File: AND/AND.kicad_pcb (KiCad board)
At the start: 2 copper layers, 33.7 x 17.8 mm, 9 parts, among them J1 Conn_01x01, J2 Conn_01x01, J3 Conn_01x01, J4 Conn_01x01, J5 Conn_01x02

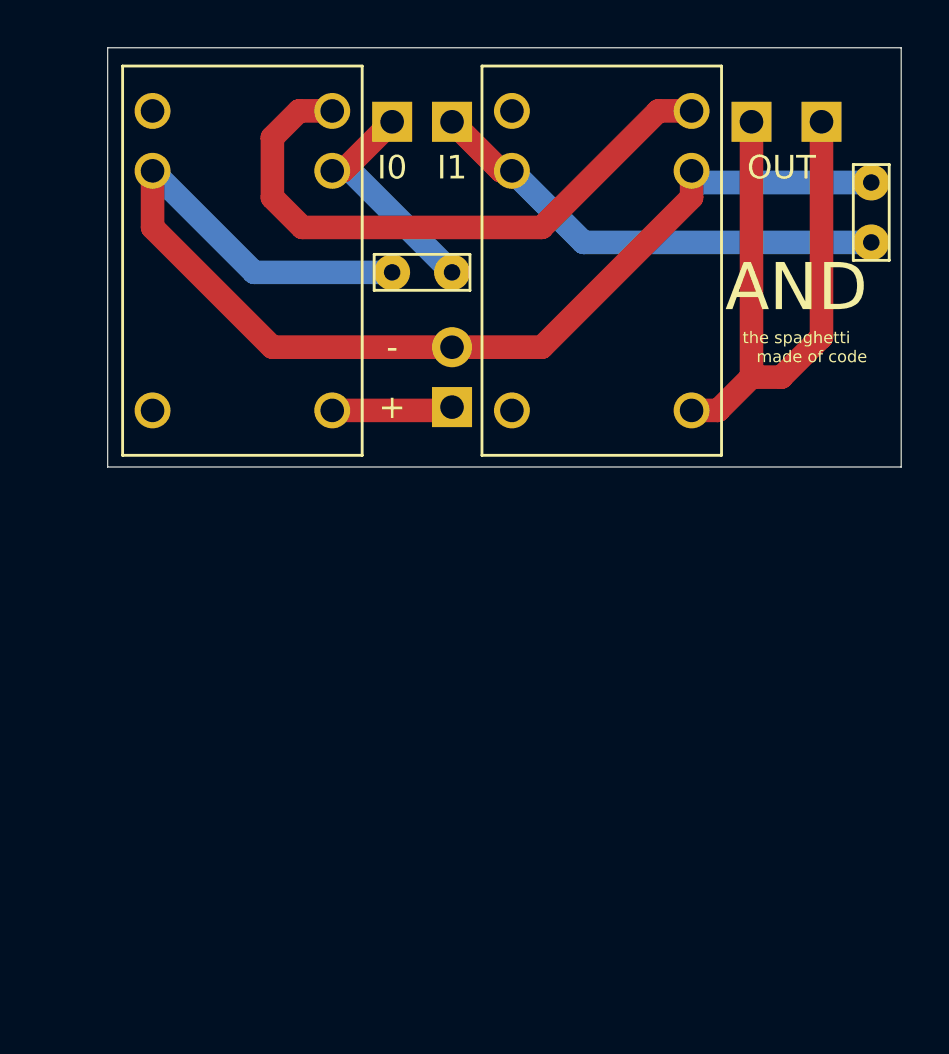
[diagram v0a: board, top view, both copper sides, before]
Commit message: Add files via upload
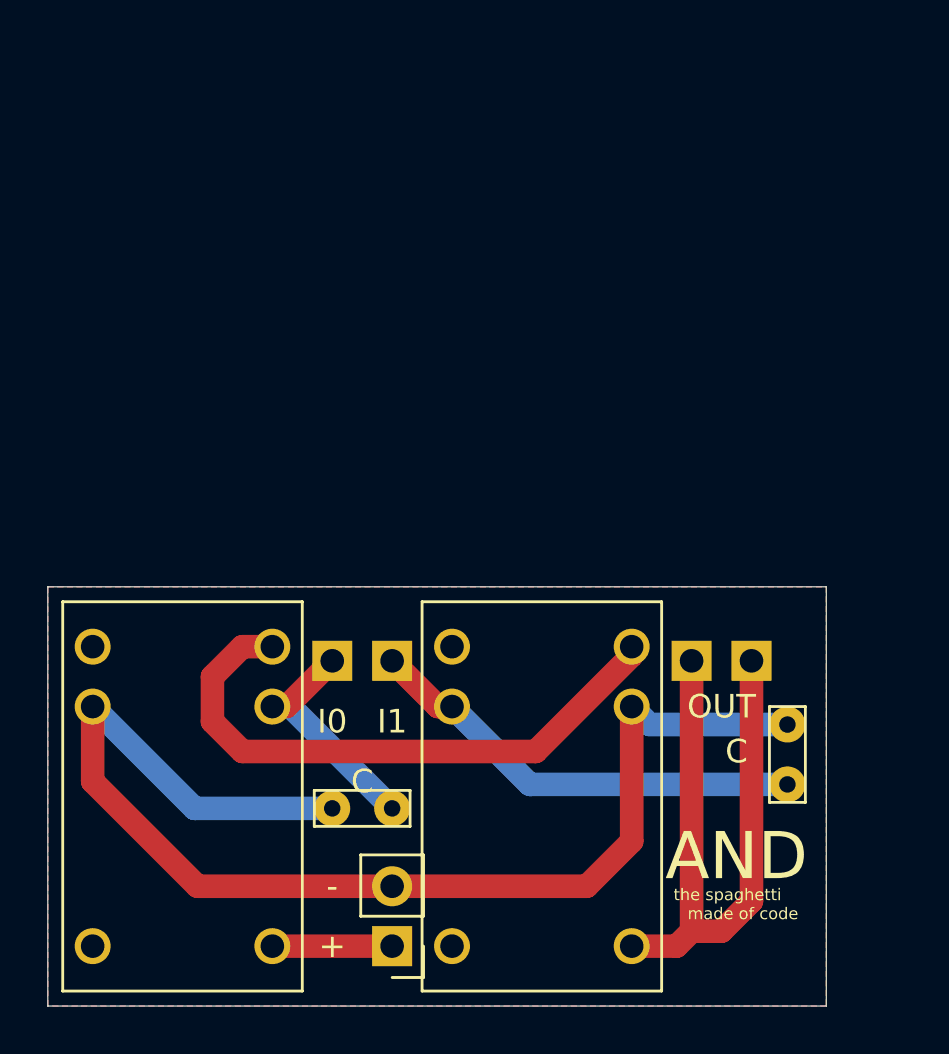
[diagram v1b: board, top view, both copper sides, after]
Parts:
- J5: moved to F.Cu
- moved C2 23.3 mm to (123.4, 127.8)
- moved J4 23.1 mm to (121.9, 125.1)
- moved J1 23.0 mm to (104.1, 125.1)
- moved J2 23.0 mm to (106.7, 125.1)
- moved J3 23.0 mm to (119.4, 125.1)
- moved J5 23.0 mm to (106.7, 137.2), turned to 180 degrees
- moved C1 22.9 mm to (106.7, 131.3)
- moved SPDT1 22.9 mm to (99.1, 129.5)
- moved SPDT2 22.9 mm to (114.3, 129.5)
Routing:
- net GND: track 50.9 -> 53.2 mm
- net Net-(C2-Pad2): track 19.9 -> 18.9 mm
- net Net-(J3-Pad1): track 26.8 -> 27.5 mm
- net +24V: track 31.0 -> 30.4 mm
- added copper zone on B.Cu, net GND
- added copper zone on F.Cu, net GND
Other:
- board size 33.7 x 17.8 mm -> 33 x 17.8 mm
- board text added: "C"
